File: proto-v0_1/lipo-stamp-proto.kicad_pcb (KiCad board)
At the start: 4 copper layers, 45.7 x 45.7 mm, 109 parts, among them Q1 Q_PMOS_GSD, U3 MCP73832-2-OT, U4 AP2112K-3.3, U5 AP9101CK6, U6 FS8205

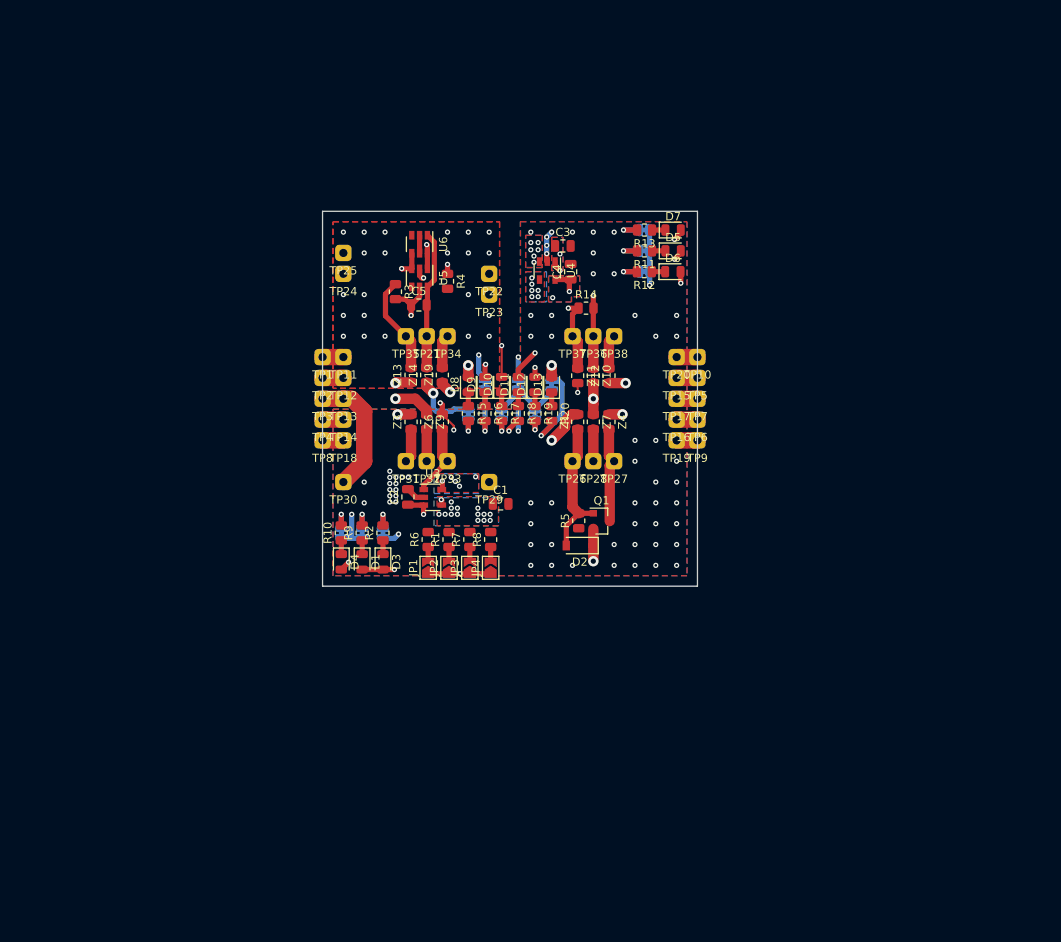
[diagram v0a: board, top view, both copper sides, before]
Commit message: Almost done, just needs back silkscreen
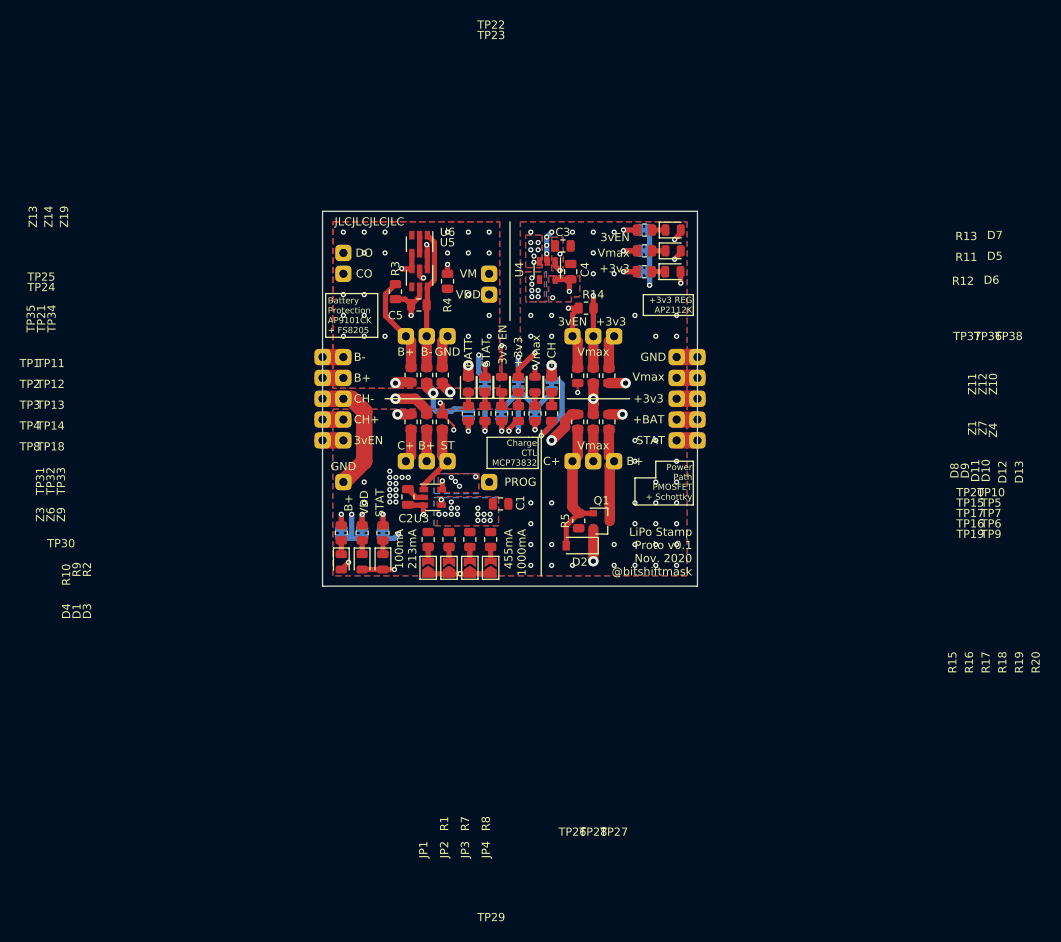
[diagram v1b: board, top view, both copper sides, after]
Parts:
- JP11: value Jumper_NC_Small -> Jumper_NO_Small; footprint Jumper:SolderJumper-2_P1.3mm_Bridged_RoundedPad1.0x1.5mm -> Jumper:SolderJumper-2_P1.3mm_Open_RoundedPad1.0x1.5mm
- turned JP11 to 90 degrees
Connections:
- JP11 pad 1: /-BATT -> Net-(JP11-Pad1)
- JP11 pad 2: Net-(JP11-Pad2) -> /-BATT
- R15 pad 2: Net-(JP11-Pad2) -> Net-(JP11-Pad1)
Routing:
- net Net-(JP11-Pad2): track 2.61 -> 0.00 mm, vias 1 -> 0
- net Net-(JP11-Pad1): track 0.00 -> 2.61 mm, vias 0 -> 1
- added copper zone on B.Cu, net Net-(R4-Pad2)
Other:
- board text added: "+3v3"
- board text added: "+3v3 REG AP2112K"
- board text added: "+BAT"
- board text added: "+CH"
- board text added: "100mA 213mA"
- board text added: "3v3 EN"
- board text added: "3vEN"
- board text added: "455mA 1000mA"
- board text added: "B+"
- board text added: "B-"
- board text added: "BATT"
- board text added: "Battery Protection AP9101CK + FS8205"
- board text added: "C+"
- board text added: "CH+"
- board text added: "CH-"
- board text added: "CO"
- board text added: "Charge CTL MCP73832"
- board text added: "DO"
- board text added: "GND"
- board text added: "JLCJLCJLCJLC"
- board text added: "LiPo Stamp Proto v0.1 Nov. 2020 @bitshiftmask"
- board text added: "PROG"
- board text added: "Power Path PMOSFET + Schottky"
- board text added: "ST"
- board text added: "STAT"
- board text added: "VDD"
- board text added: "VM"
- board text added: "Vmax"
